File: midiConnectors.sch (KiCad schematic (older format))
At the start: 9 parts

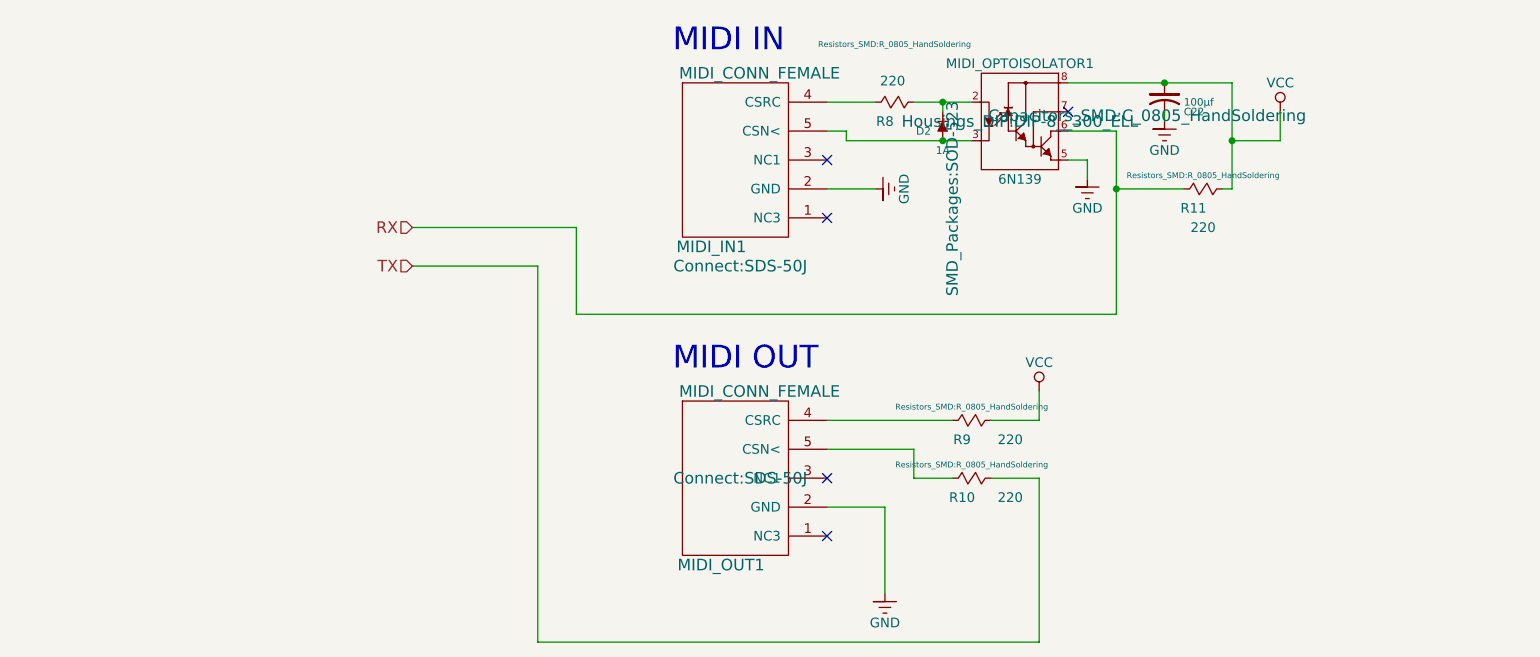
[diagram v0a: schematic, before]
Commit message: UPDATEUPDATES!!!
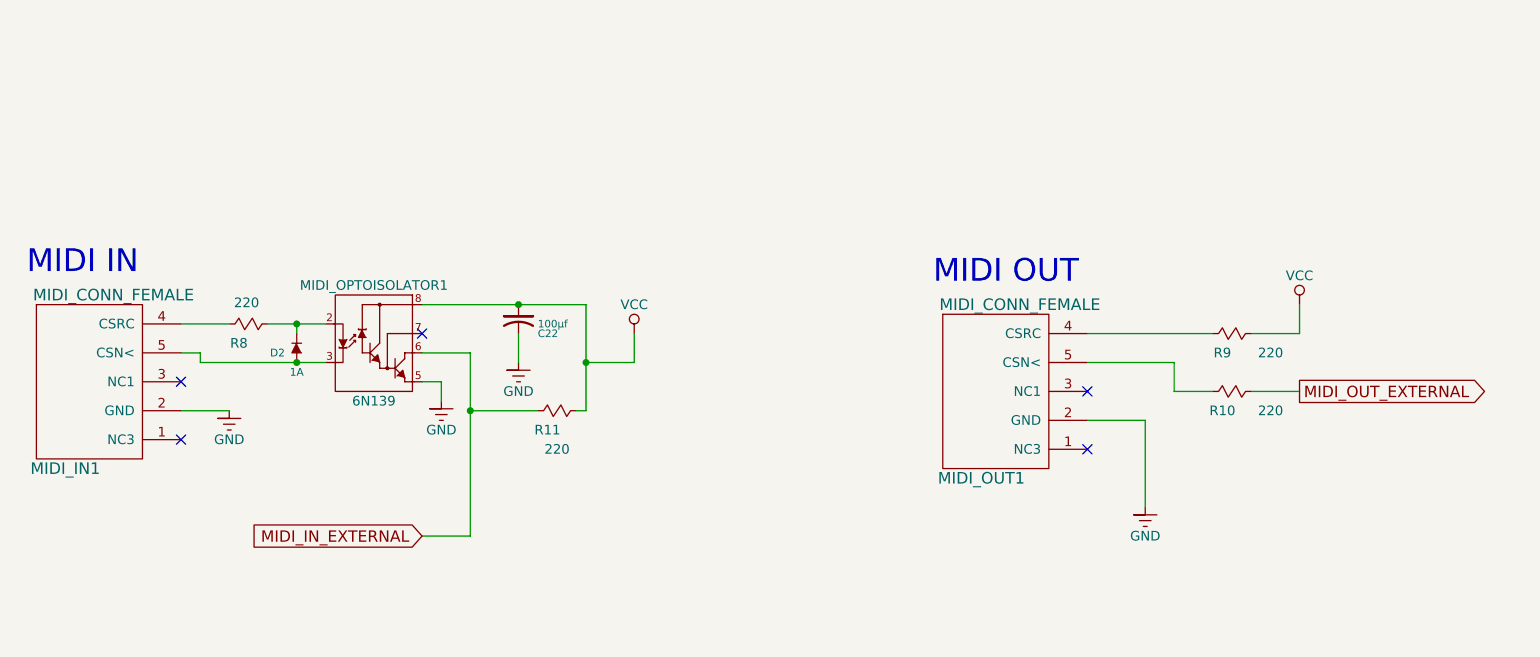
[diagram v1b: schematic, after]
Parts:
- MIDI_IN1, MIDI_OUT1: footprint Connect:SDS-50J -> Zetaohm:MIDI_Wire_Connector
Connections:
- net RX renamed MIDI_IN_EXTERNAL
- net TX renamed MIDI_OUT_EXTERNAL
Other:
- moved on the sheet: C22, D2, MIDI_IN1, MIDI_OPTOISOLATOR1, MIDI_OUT1, R10, R11, R8, R9

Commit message: Updating footprints
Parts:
- C22: footprint Capacitors_SMD:C_0805_HandSoldering -> Capacitors_SMD:C_0603_HandSoldering
- MIDI_OPTOISOLATOR1: footprint Housings_DIP:DIP-8__300_ELL -> SMD_Packages:DIP-8_SMD
- MIDI_OUT1: footprint Zetaohm:MIDI_Wire_Connector -> SMD_Packages:DIP-8_SMD
- R10, R11, R8, R9: footprint Resistors_SMD:R_0805_HandSoldering -> Resistors_SMD:R_0603_HandSoldering
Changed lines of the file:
@@
 $Descr A4 11693 8268
 encoding utf-8
-Sheet 7 8
+Sheet 7 7
 Title ""
 Date ""
@@
 F 0 "MIDI_OUT1" H 7300 3300 60  0000 C CNN
 F 1 "MIDI_CONN_FEMALE" H 7500 4200 60  0000 C CNN
-F 2 "Zetaohm:MIDI_Wire_Connector" H 7400 3750 60  0001 C CNN
+F 2 "SMD_Packages:DIP-8_SMD" H 7400 3750 60  0001 C CNN
 F 3 "" H 7400 3750 60  0000 C CNN
 	1    7400 3750
@@
 F 0 "MIDI_OPTOISOLATOR1" H 4150 3800 50  0000 C CNN
 F 1 "6N139" H 4150 3200 50  0000 C CNN
-F 2 "Housings_DIP:DIP-8__300_ELL" H 4150 3500 60  0001 C CNN
+F 2 "SMD_Packages:DIP-8_SMD" H 4150 3500 60  0001 C CNN
 F 3 "" H 4150 3500 60  0000 C CNN
 	1    4150 3500
@@
 F 0 "R8" V 3600 3350 50  0000 C CNN
 F 1 "220" V 3390 3390 50  0000 C CNN
-F 2 "Resistors_SMD:R_0805_HandSoldering" V 3200 3400 30  0001 C CNN
+F 2 "Resistors_SMD:R_0603_HandSoldering" V 3200 3400 30  0001 C CNN
 F 3 "" H 3500 3400 30  0000 C CNN
 	1    3500 3400
@@
 NoConn ~ 3150 4000
 $Comp
-L GND-RESCUE-afx-01 #PWR0122
+L GND-RESCUE-afx-01 #PWR098
 U 1 1 557B4E62
 P 3400 3850
-F 0 "#PWR0122" H 3400 3600 50  0001 C CNN
+F 0 "#PWR098" H 3400 3600 50  0001 C CNN
 F 1 "GND" H 3400 3700 50  0000 C CNN
 F 2 "" H 3400 3850 60  0000 C CNN
@@
 F 0 "C22" H 5000 3350 39  0000 L CNN
 F 1 "100µf" H 5000 3400 39  0000 L CNN
-F 2 "Capacitors_SMD:C_0805_HandSoldering" H 4810 3330 60  0001 C CNN
+F 2 "Capacitors_SMD:C_0603_HandSoldering" H 4810 3330 60  0001 C CNN
 F 3 "" H 4900 3400 60  0000 C CNN
 	1    4900 3400
@@
 $EndComp
 $Comp
-L GND-RESCUE-afx-01 #PWR0123
+L GND-RESCUE-afx-01 #PWR099
 U 1 1 557B4E70
 P 4900 3600
-F 0 "#PWR0123" H 4900 3350 50  0001 C CNN
+F 0 "#PWR099" H 4900 3350 50  0001 C CNN
 F 1 "GND" H 4900 3450 50  0000 C CNN
 F 2 "" H 4900 3600 60  0000 C CNN
@@
 F 0 "R11" V 5200 3800 50  0000 C CNN
 F 1 "220" V 5300 3850 50  0000 C CNN
-F 2 "Resistors_SMD:R_0805_HandSoldering" V 5030 3850 30  0001 C CNN
+F 2 "Resistors_SMD:R_0603_HandSoldering" V 5030 3850 30  0001 C CNN
 F 3 "" H 5100 3850 30  0000 C CNN
 	1    5100 3850
@@
 Connection ~ 5250 3600
 $Comp
-L VCC #PWR0124
+L VCC #PWR0100
 U 1 1 557B4E8A
 P 5500 3450
-F 0 "#PWR0124" H 5500 3300 50  0001 C CNN
+F 0 "#PWR0100" H 5500 3300 50  0001 C CNN
 F 1 "VCC" H 5500 3600 50  0000 C CNN
 F 2 "" H 5500 3450 60  0000 C CNN
@@
 $EndComp
 $Comp
-L GND-RESCUE-afx-01 #PWR0125
+L GND-RESCUE-afx-01 #PWR0101
 U 1 1 557B4E90
 P 4500 3800
-F 0 "#PWR0125" H 4500 3550 50  0001 C CNN
+F 0 "#PWR0101" H 4500 3550 50  0001 C CNN
 F 1 "GND" H 4500 3650 50  0000 C CNN
 F 2 "" H 4500 3800 60  0000 C CNN
@@
 F 0 "R9" V 8700 3400 50  0000 C CNN
 F 1 "220" V 8700 3650 50  0000 C CNN
-F 2 "Resistors_SMD:R_0805_HandSoldering" V 8530 3450 30  0001 C CNN
+F 2 "Resistors_SMD:R_0603_HandSoldering" V 8530 3450 30  0001 C CNN
 F 3 "" H 8600 3450 30  0000 C CNN
 	1    8600 3450
@@
 	7850 3450 8500 3450
 $Comp
-L VCC #PWR0126
+L VCC #PWR0102
 U 1 1 557B4EA2
 P 8950 3300
-F 0 "#PWR0126" H 8950 3150 50  0001 C CNN
+F 0 "#PWR0102" H 8950 3150 50  0001 C CNN
 F 1 "VCC" H 8950 3450 50  0000 C CNN
 F 2 "" H 8950 3300 60  0000 C CNN
@@
 F 0 "R10" V 8700 3700 50  0000 C CNN
 F 1 "220" V 8700 3950 50  0000 C CNN
-F 2 "Resistors_SMD:R_0805_HandSoldering" V 8530 3750 30  0001 C CNN
+F 2 "Resistors_SMD:R_0603_HandSoldering" V 8530 3750 30  0001 C CNN
 F 3 "" H 8600 3750 30  0000 C CNN
 	1    8600 3750
@@
 	8150 3900 8150 4350
 $Comp
-L GND-RESCUE-afx-01 #PWR0127
+L GND-RESCUE-afx-01 #PWR0103
 U 1 1 557B4EB7
 P 8150 4350
-F 0 "#PWR0127" H 8150 4100 50  0001 C CNN
+F 0 "#PWR0103" H 8150 4100 50  0001 C CNN
 F 1 "GND" H 8150 4200 50  0000 C CNN
 F 2 "" H 8150 4350 60  0000 C CNN

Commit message: Populating pcb file
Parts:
- MIDI_OUT1: footprint SMD_Packages:DIP-8_SMD -> Zetaohm:MIDI_Wire_Connector
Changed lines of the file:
@@
 F 0 "MIDI_OUT1" H 7300 3300 60  0000 C CNN
 F 1 "MIDI_CONN_FEMALE" H 7500 4200 60  0000 C CNN
-F 2 "SMD_Packages:DIP-8_SMD" H 7400 3750 60  0001 C CNN
+F 2 "Zetaohm:MIDI_Wire_Connector" H 7400 3750 60  0001 C CNN
 F 3 "" H 7400 3750 60  0000 C CNN
 	1    7400 3750
@@
 NoConn ~ 3150 4000
 $Comp
-L GND-RESCUE-afx-01 #PWR098
+L GND-RESCUE-afx-01 #PWR103
 U 1 1 557B4E62
 P 3400 3850
-F 0 "#PWR098" H 3400 3600 50  0001 C CNN
+F 0 "#PWR103" H 3400 3600 50  0001 C CNN
 F 1 "GND" H 3400 3700 50  0000 C CNN
 F 2 "" H 3400 3850 60  0000 C CNN
@@
 $EndComp
 $Comp
-L GND-RESCUE-afx-01 #PWR099
+L GND-RESCUE-afx-01 #PWR101
 U 1 1 557B4E70
 P 4900 3600
-F 0 "#PWR099" H 4900 3350 50  0001 C CNN
+F 0 "#PWR101" H 4900 3350 50  0001 C CNN
 F 1 "GND" H 4900 3450 50  0000 C CNN
 F 2 "" H 4900 3600 60  0000 C CNN
@@
 Connection ~ 5250 3600
 $Comp
-L VCC #PWR0100
+L VCC #PWR100
 U 1 1 557B4E8A
 P 5500 3450
-F 0 "#PWR0100" H 5500 3300 50  0001 C CNN
+F 0 "#PWR100" H 5500 3300 50  0001 C CNN
 F 1 "VCC" H 5500 3600 50  0000 C CNN
 F 2 "" H 5500 3450 60  0000 C CNN
@@
 $EndComp
 $Comp
-L GND-RESCUE-afx-01 #PWR0101
+L GND-RESCUE-afx-01 #PWR102
 U 1 1 557B4E90
 P 4500 3800
-F 0 "#PWR0101" H 4500 3550 50  0001 C CNN
+F 0 "#PWR102" H 4500 3550 50  0001 C CNN
 F 1 "GND" H 4500 3650 50  0000 C CNN
 F 2 "" H 4500 3800 60  0000 C CNN
@@
 	7850 3450 8500 3450
 $Comp
-L VCC #PWR0102
+L VCC #PWR99
 U 1 1 557B4EA2
 P 8950 3300
-F 0 "#PWR0102" H 8950 3150 50  0001 C CNN
+F 0 "#PWR99" H 8950 3150 50  0001 C CNN
 F 1 "VCC" H 8950 3450 50  0000 C CNN
 F 2 "" H 8950 3300 60  0000 C CNN
@@
 	8150 3900 8150 4350
 $Comp
-L GND-RESCUE-afx-01 #PWR0103
+L GND-RESCUE-afx-01 #PWR104
 U 1 1 557B4EB7
 P 8150 4350
-F 0 "#PWR0103" H 8150 4100 50  0001 C CNN
+F 0 "#PWR104" H 8150 4100 50  0001 C CNN
 F 1 "GND" H 8150 4200 50  0000 C CNN
 F 2 "" H 8150 4350 60  0000 C CNN
